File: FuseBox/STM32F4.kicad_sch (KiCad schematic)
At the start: 25 parts, among them J1 61301611121, J2 61301611121, J3 61301611121, J4 61301611121, J5 61301611121, U1 STM32F407VGTx

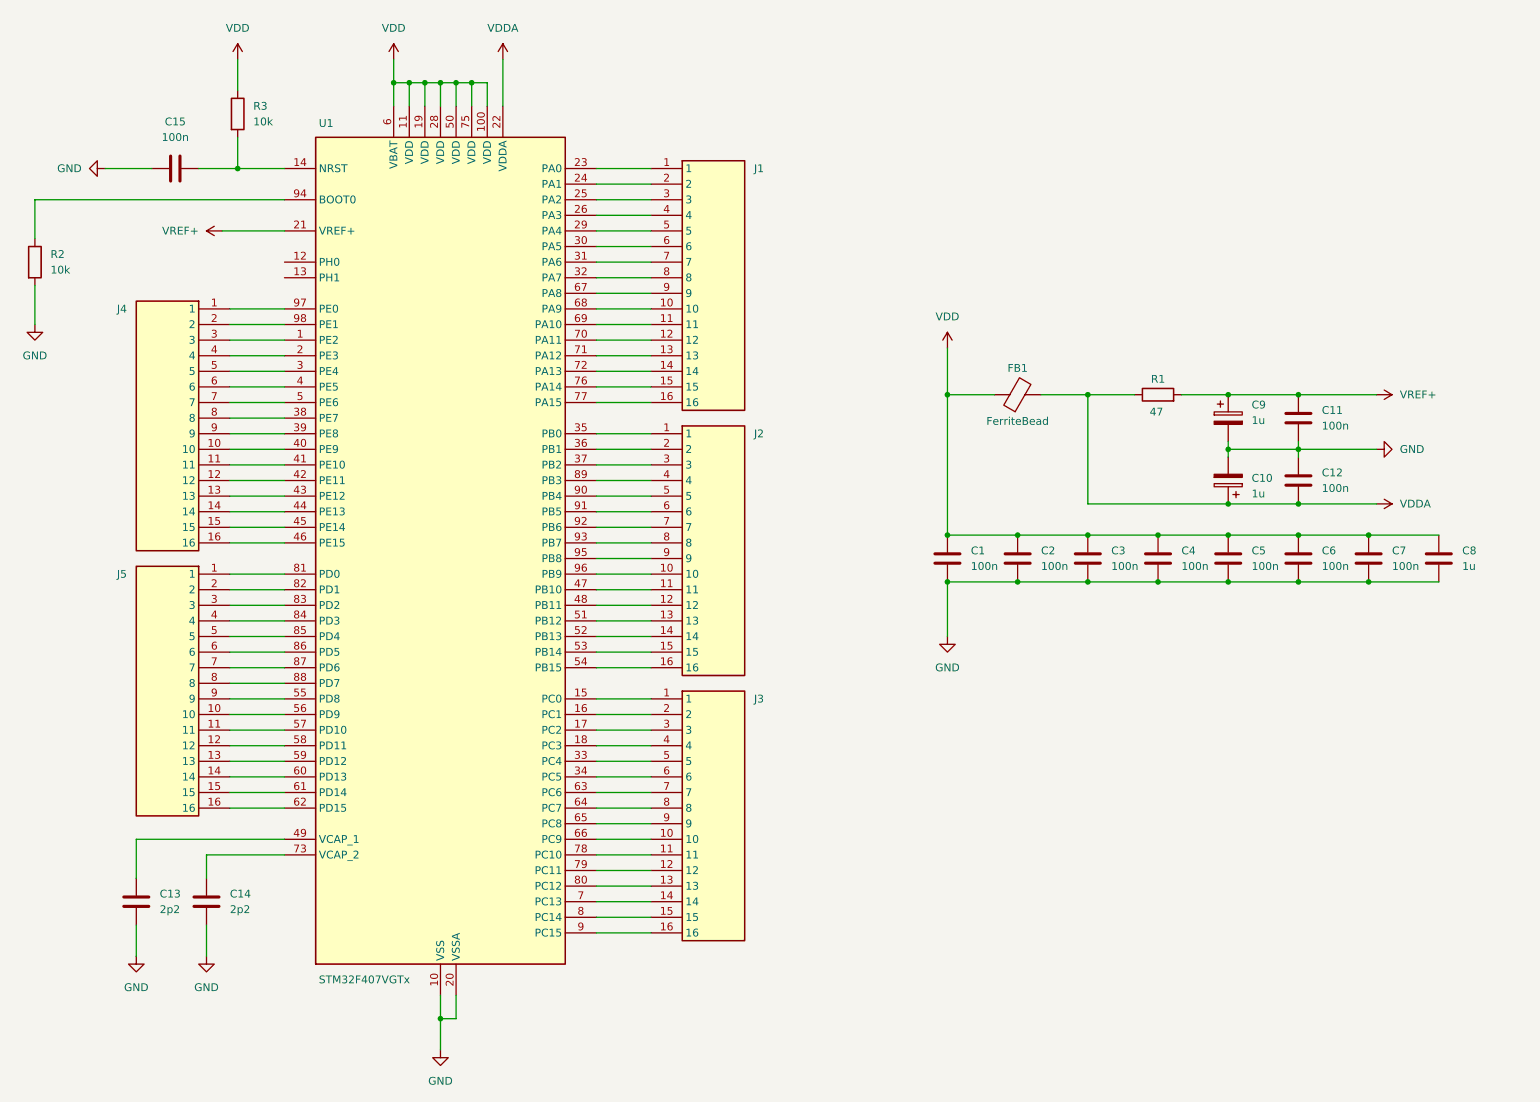
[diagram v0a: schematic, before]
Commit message: some foo
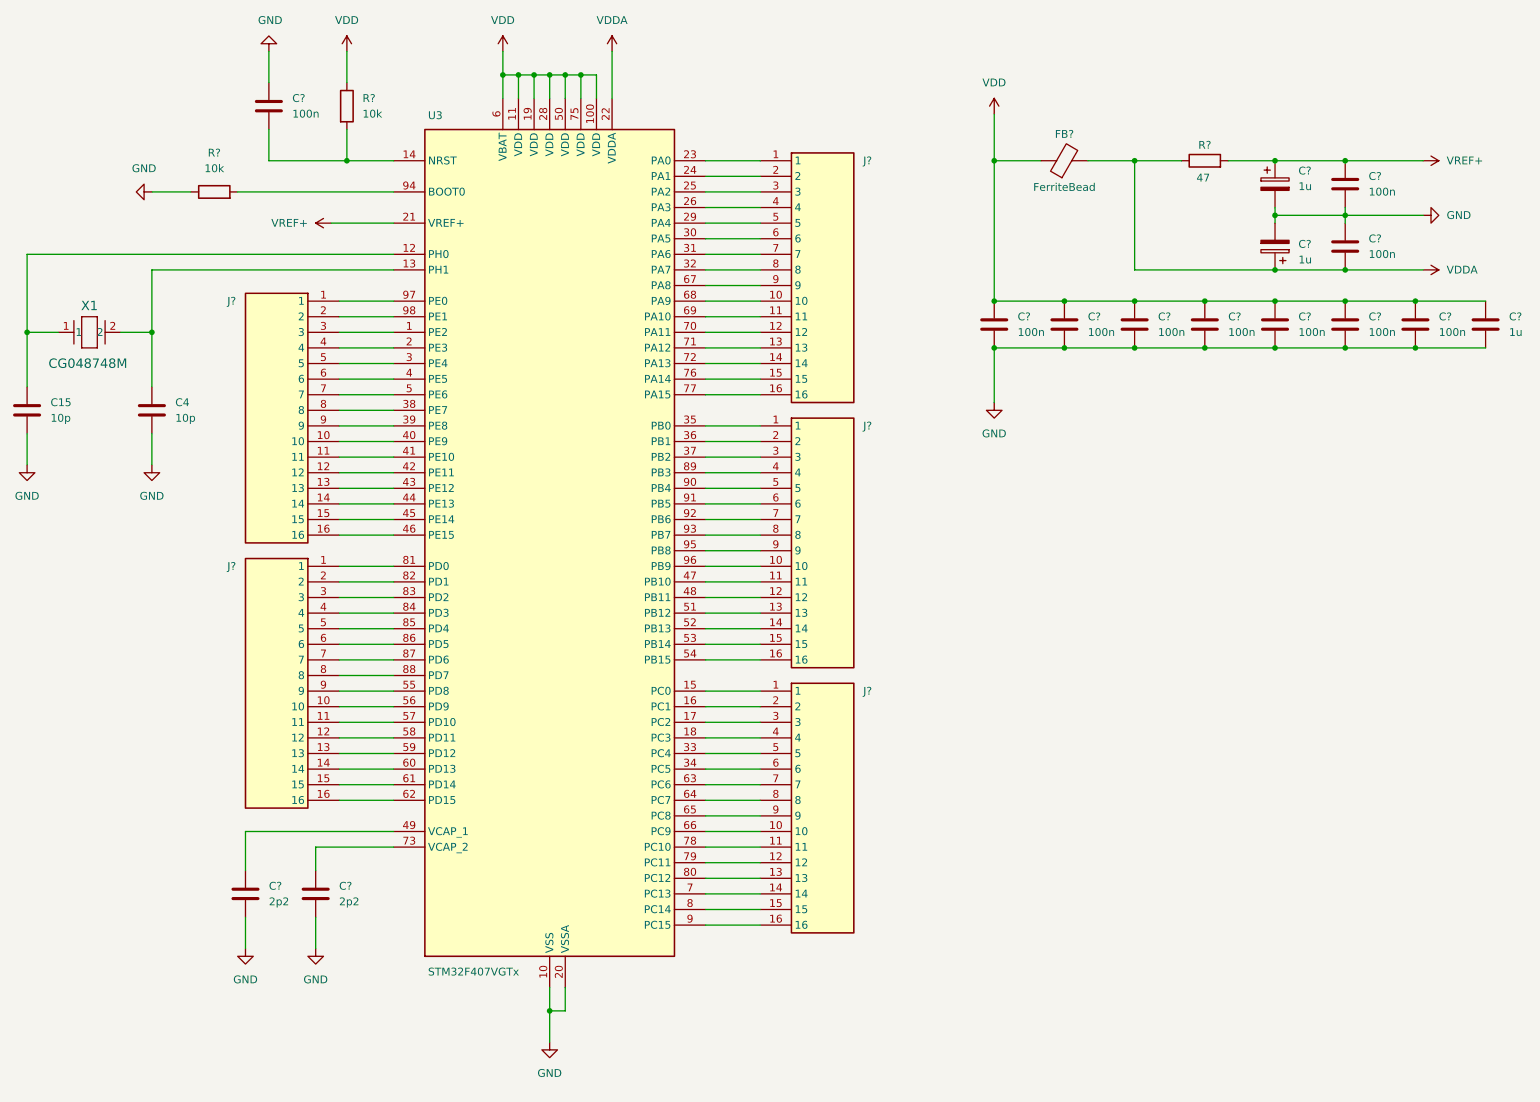
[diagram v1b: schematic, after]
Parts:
- added C4: 10p, symbol Device:C
- added X1: CG048748M, Custom:CG048748M, symbol Custom:CG048748M
- renumbered C1 to C?, C8 to C?, C9 to C?, C15 to C?, C2 to C?, C11 to C?, C12 to C?, C6 to C?, C14 to C?, C10 to C?, C3 to C?, C5 to C?, C13 to C?, C4 to C?, C7 to C?, FB1 to FB?, J4 to J?, J2 to J?, J3 to J?, J1 to J?, J5 to J?, R1 to R?, R2 to R?, R3 to R?, U1 to U3
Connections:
- net GND: now also C?.2, R?.1, C4.1; no longer R?.2
- net at U3.12 (PH0): now also C?.2, X1.1
- net at U3.13 (PH1): now also C4.2, X1.2
- net at R?.2, U3.14 (NRST): now also C?.1; no longer C?.2
- net at U3.94 (BOOT0): now also R?.2; no longer R?.1
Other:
- moved on the sheet: C15, C?, FB?, J?, R?, U3
